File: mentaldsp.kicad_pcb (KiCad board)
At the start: 2 copper layers, 125 x 35 mm, 14 parts, among them J5 NEMA Conn, J7 NEMA Conn, J8 NEMA Conn, J9 Barrel_Jack_Switch, U6 ESP32-S3-SUPERMINI, U7 TMC2209_N0, U8 TMC2209_N1, U9 TMC2209_N2

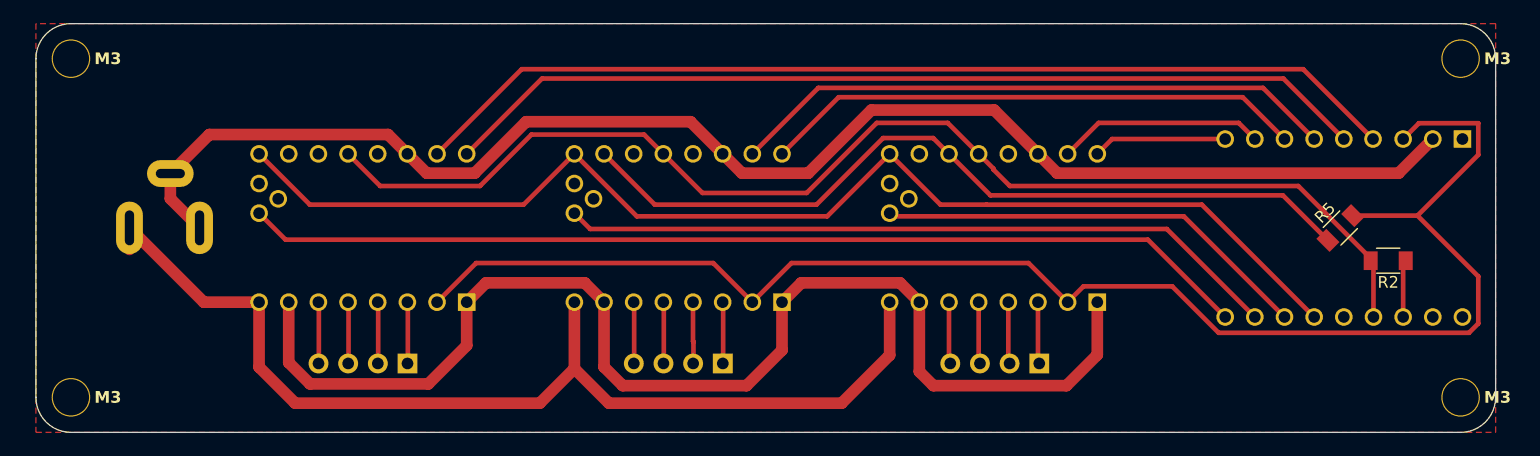
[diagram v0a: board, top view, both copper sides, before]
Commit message: decoupling
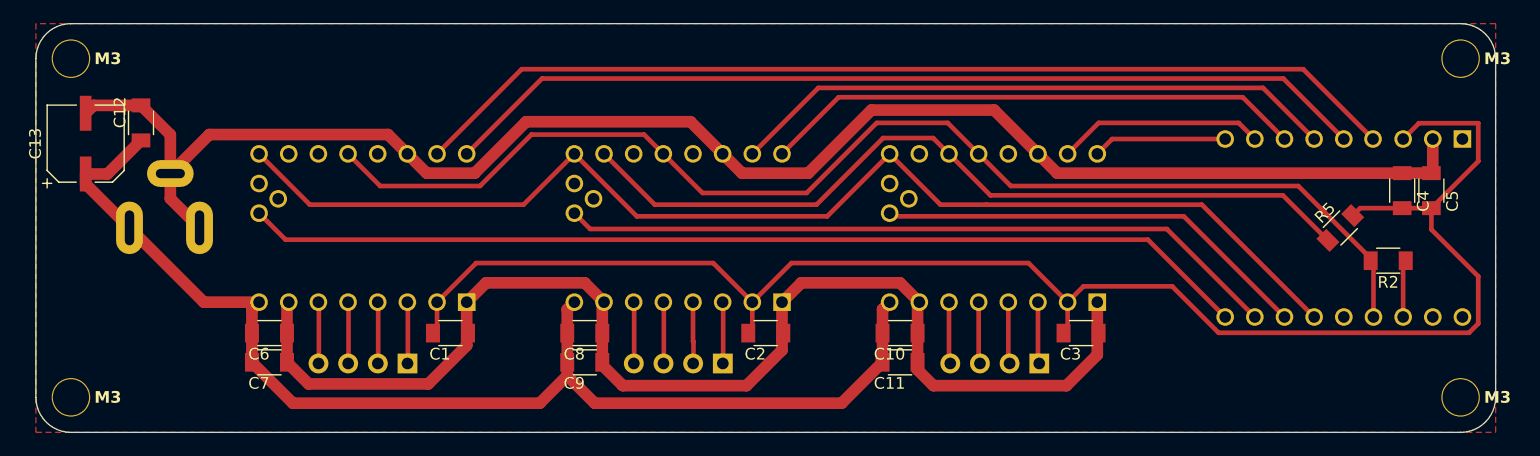
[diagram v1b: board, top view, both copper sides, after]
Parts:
- added C1: 100n, PCM_fab:C_1206, F.Cu at (135.5, 126.5)
- added C10: 100n, PCM_fab:C_1206, F.Cu at (174.0, 126.5)
- added C11: 10u, PCM_fab:C_1206, F.Cu at (174.0, 129.0)
- added C12: 100n, PCM_fab:C_1206, F.Cu at (109.0, 108.5)
- added C13: 220u, PCM_fab:CP_Elec_100uF_Panasonic_EEE-FN1E101UL, F.Cu at (104.3, 110.3)
- added C2: 100n, PCM_fab:C_1206, F.Cu at (162.5, 126.5)
- added C3: 100n, PCM_fab:C_1206, F.Cu at (189.5, 126.5)
- added C4: 100n, PCM_fab:C_1206, F.Cu at (217.0, 114.3)
- added C5: 10u, PCM_fab:C_1206, F.Cu at (219.5, 114.3)
- added C6: 100n, PCM_fab:C_1206, F.Cu at (120.0, 126.5)
- added C7: 10u, PCM_fab:C_1206, F.Cu at (120.0, 129.0)
- added C8: 100n, PCM_fab:C_1206, F.Cu at (147.0, 126.5)
- added C9: 10u, PCM_fab:C_1206, F.Cu at (147.0, 129.0)
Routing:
- net GND: track 232.5 -> 246.5 mm
- net +12V: track 90.8 -> 102.0 mm
- net +3.3V: track 201.4 -> 210.8 mm
